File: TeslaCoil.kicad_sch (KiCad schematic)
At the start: 36 parts, among them J1 Screw_Terminal_01x03, J2 Screw_Terminal_01x02, J3 Screw_Terminal_01x02, Q1 Q_NIGBT_GCE, Q2 Q_NIGBT_GCE, U1 UCC27712D, U2 L78L15_SO8, U3 ZC323000, U4 HT7533-1-SOT89

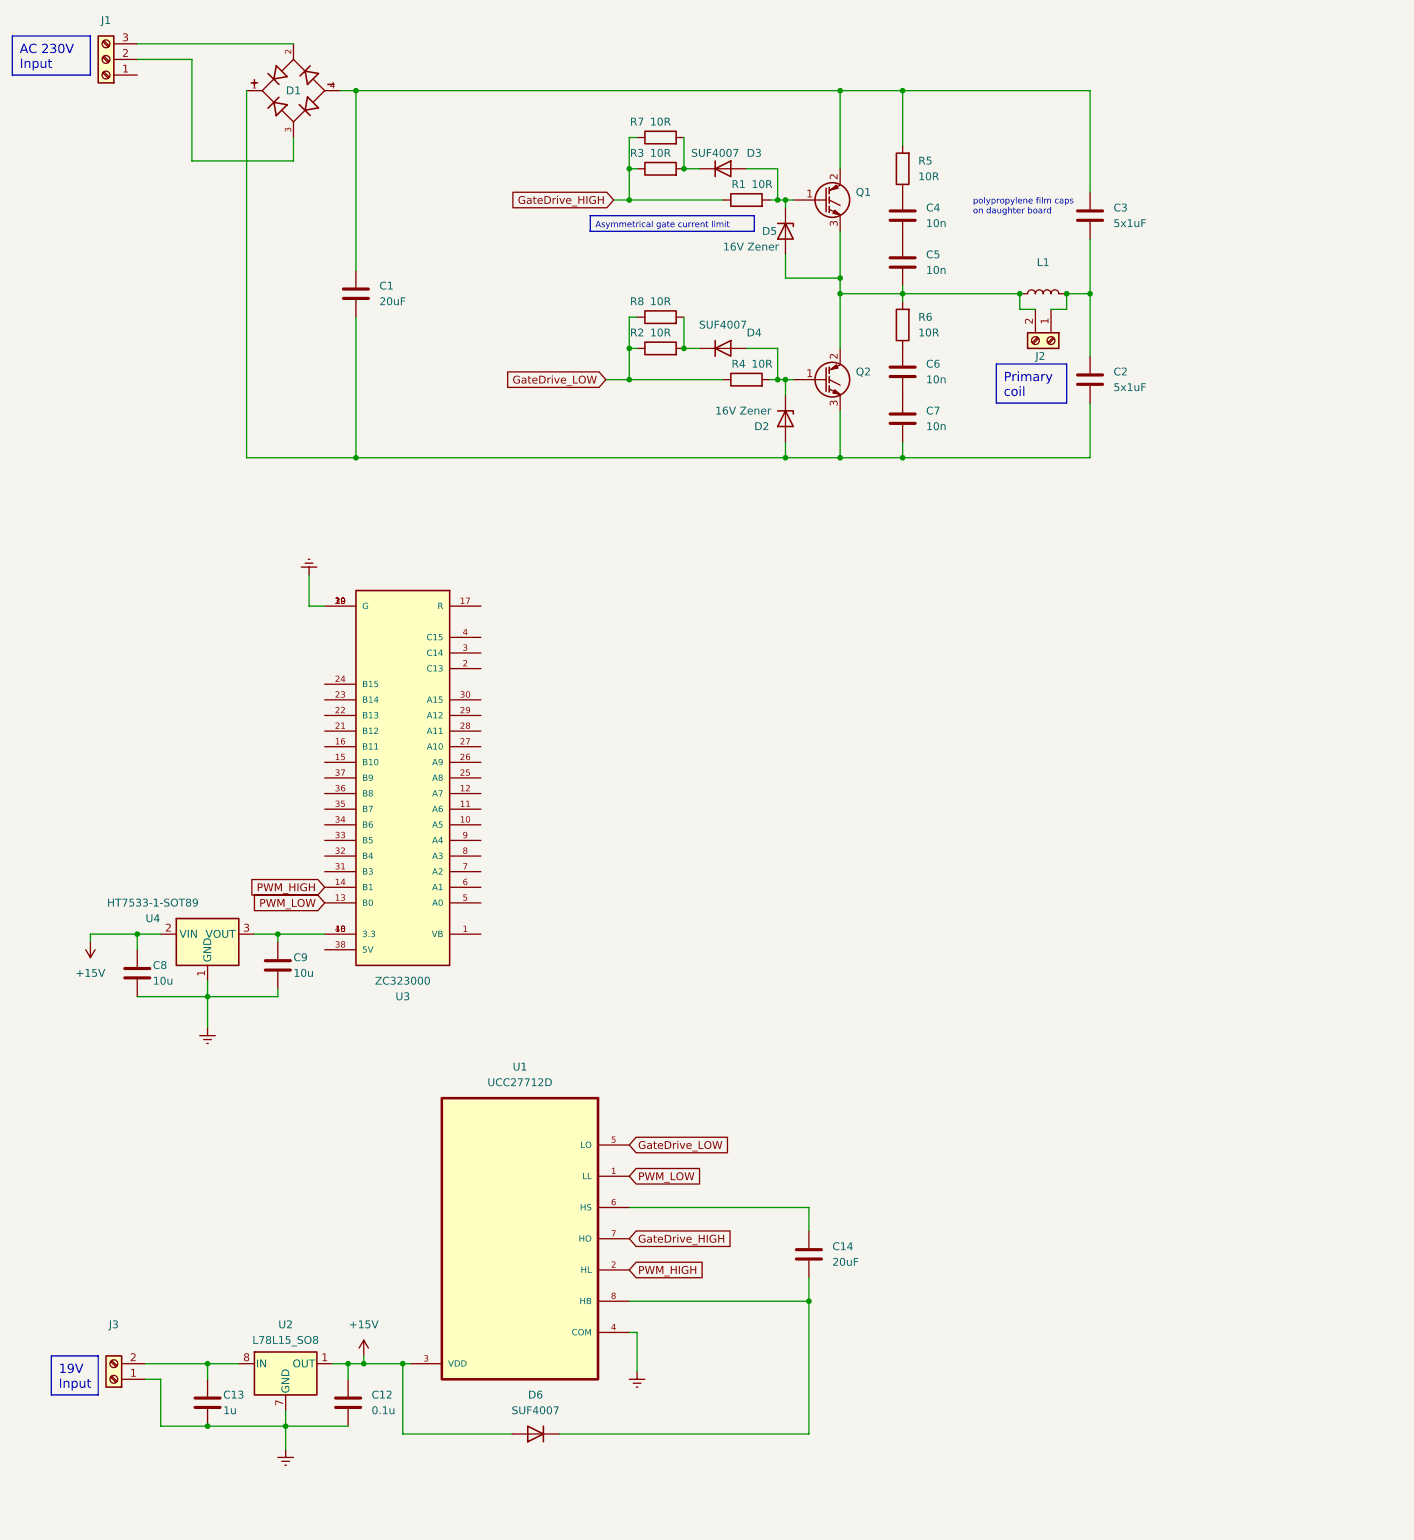
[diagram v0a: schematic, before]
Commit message: layout mockup
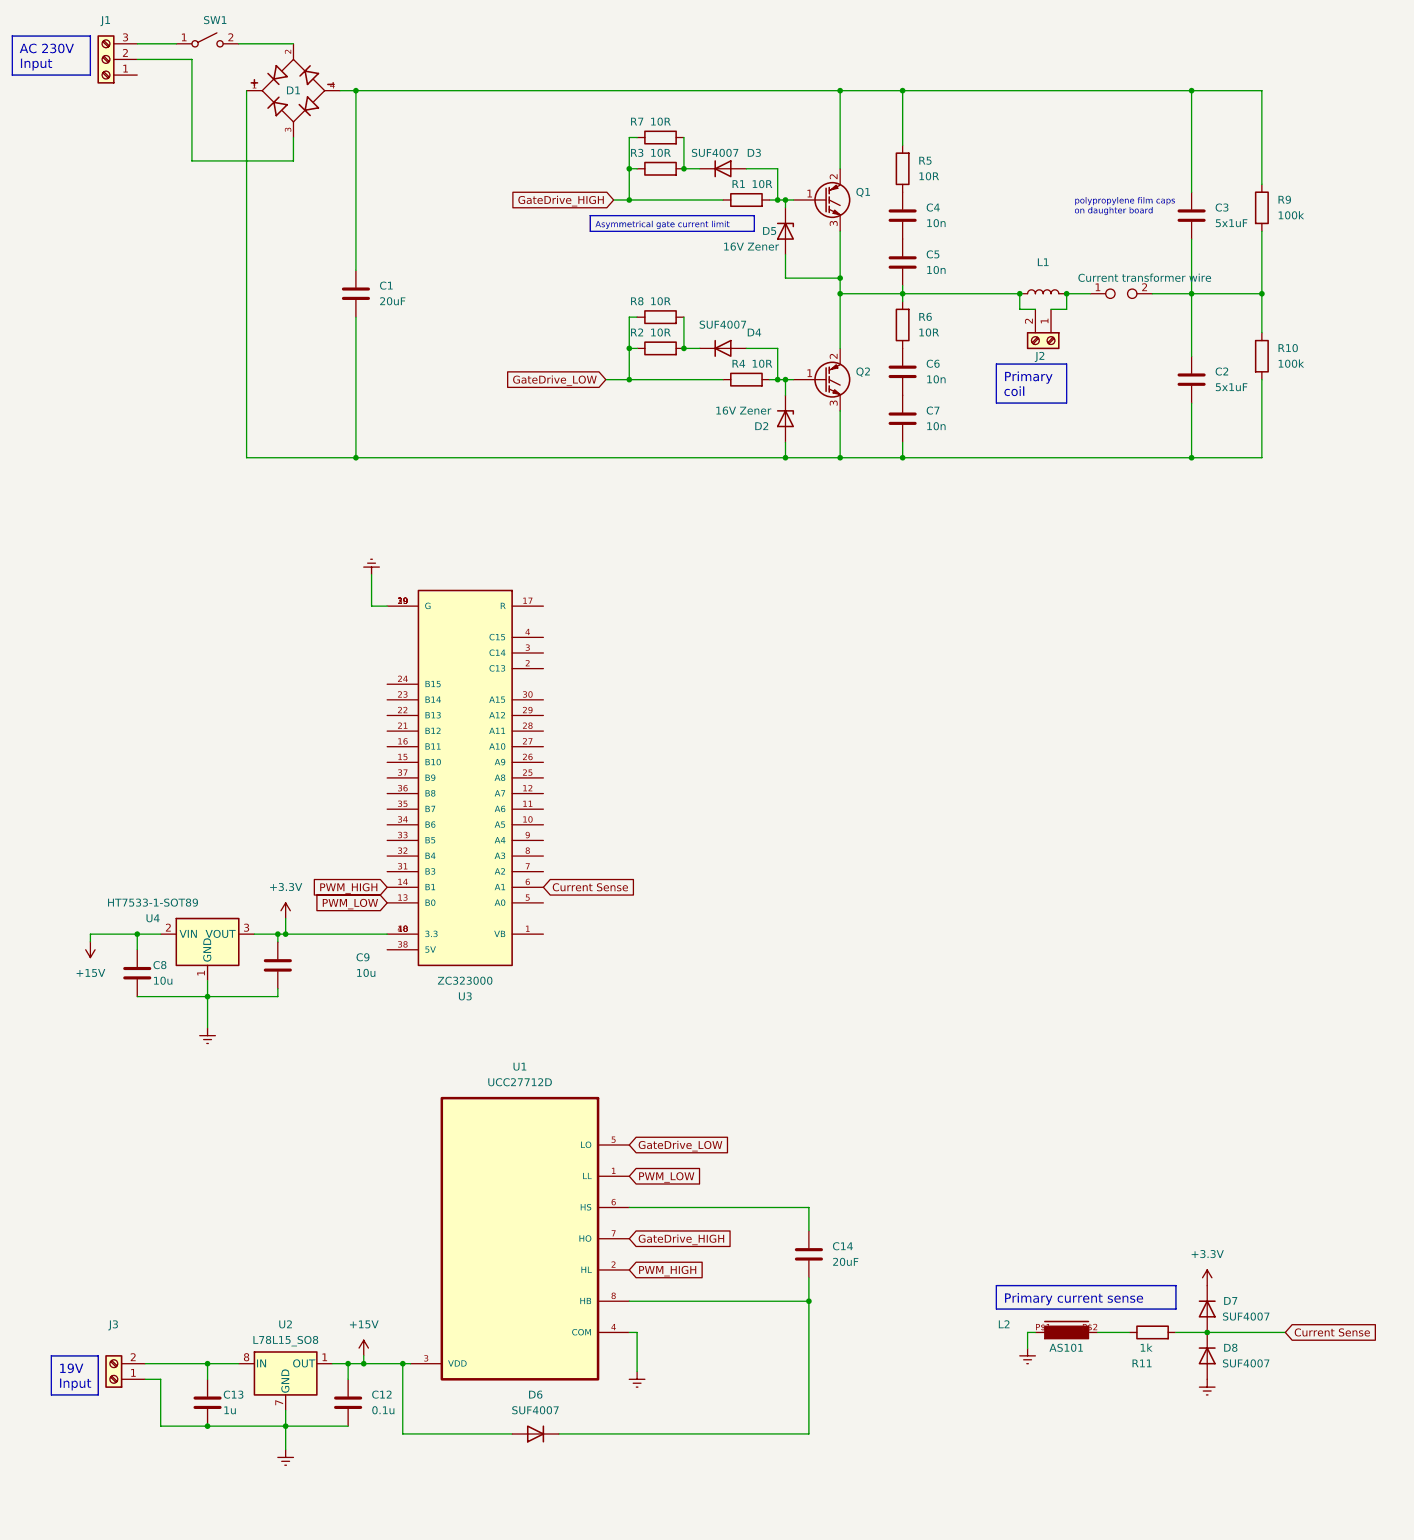
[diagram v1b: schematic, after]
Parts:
- added D7, D8: SUF4007, Diode_SMD:D_MELF_Handsoldering, symbol Diode:SM516
- added L2: AS101, Snapeda:ASM-010_ASM-010, symbol Snapeda_kicad_sym:ASM-010
- added R10, R9: 100k, Resistor_THT:R_Axial_DIN0207_L6.3mm_D2.5mm_P7.62mm_Horizontal, symbol Device:R
- added R11: 1k, Resistor_THT:R_Axial_DIN0207_L6.3mm_D2.5mm_P7.62mm_Horizontal, symbol Device:R
- added SW1: SW_SPST, symbol Switch:SW_SPST
- added TP1: Current transformer wire, TestPoint:TestPoint_Bridge_Pitch7.62mm_Drill1.3mm, symbol Connector:TestPoint_2Pole
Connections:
- net Earth: now also D8.2 (A), L2.P$1
- net at C1.2, C2.2, C7.2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: now also R10.2
- net at D1.2: now also SW1.2 (B); no longer J1.3 (Pin_3)
- net at C1.1, C3.1, D1.4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: now also R9.1
- net +3.3V: now reaches C9.1, U3.18 (3.3), U3.40 (3.3), U4.3 (VOUT)
- net +3.3V: now also D7.1 (K)
- net at J2.1 (Pin_1), L1.2: now also TP1.1; no longer C2.1, C3.2
- net Current Sense: now reaches U3.6 (A1)
- net Current Sense: now also D7.2 (A), D8.1 (K), R11.2
- new net: L2.P$2, R11.1
- new net: C2.1, C3.2, R10.1, R9.2, TP1.2
- new net: J1.3 (Pin_3), SW1.1 (A)
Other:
- moved on the sheet: C2, C3, U3

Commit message: layout 2nd rev
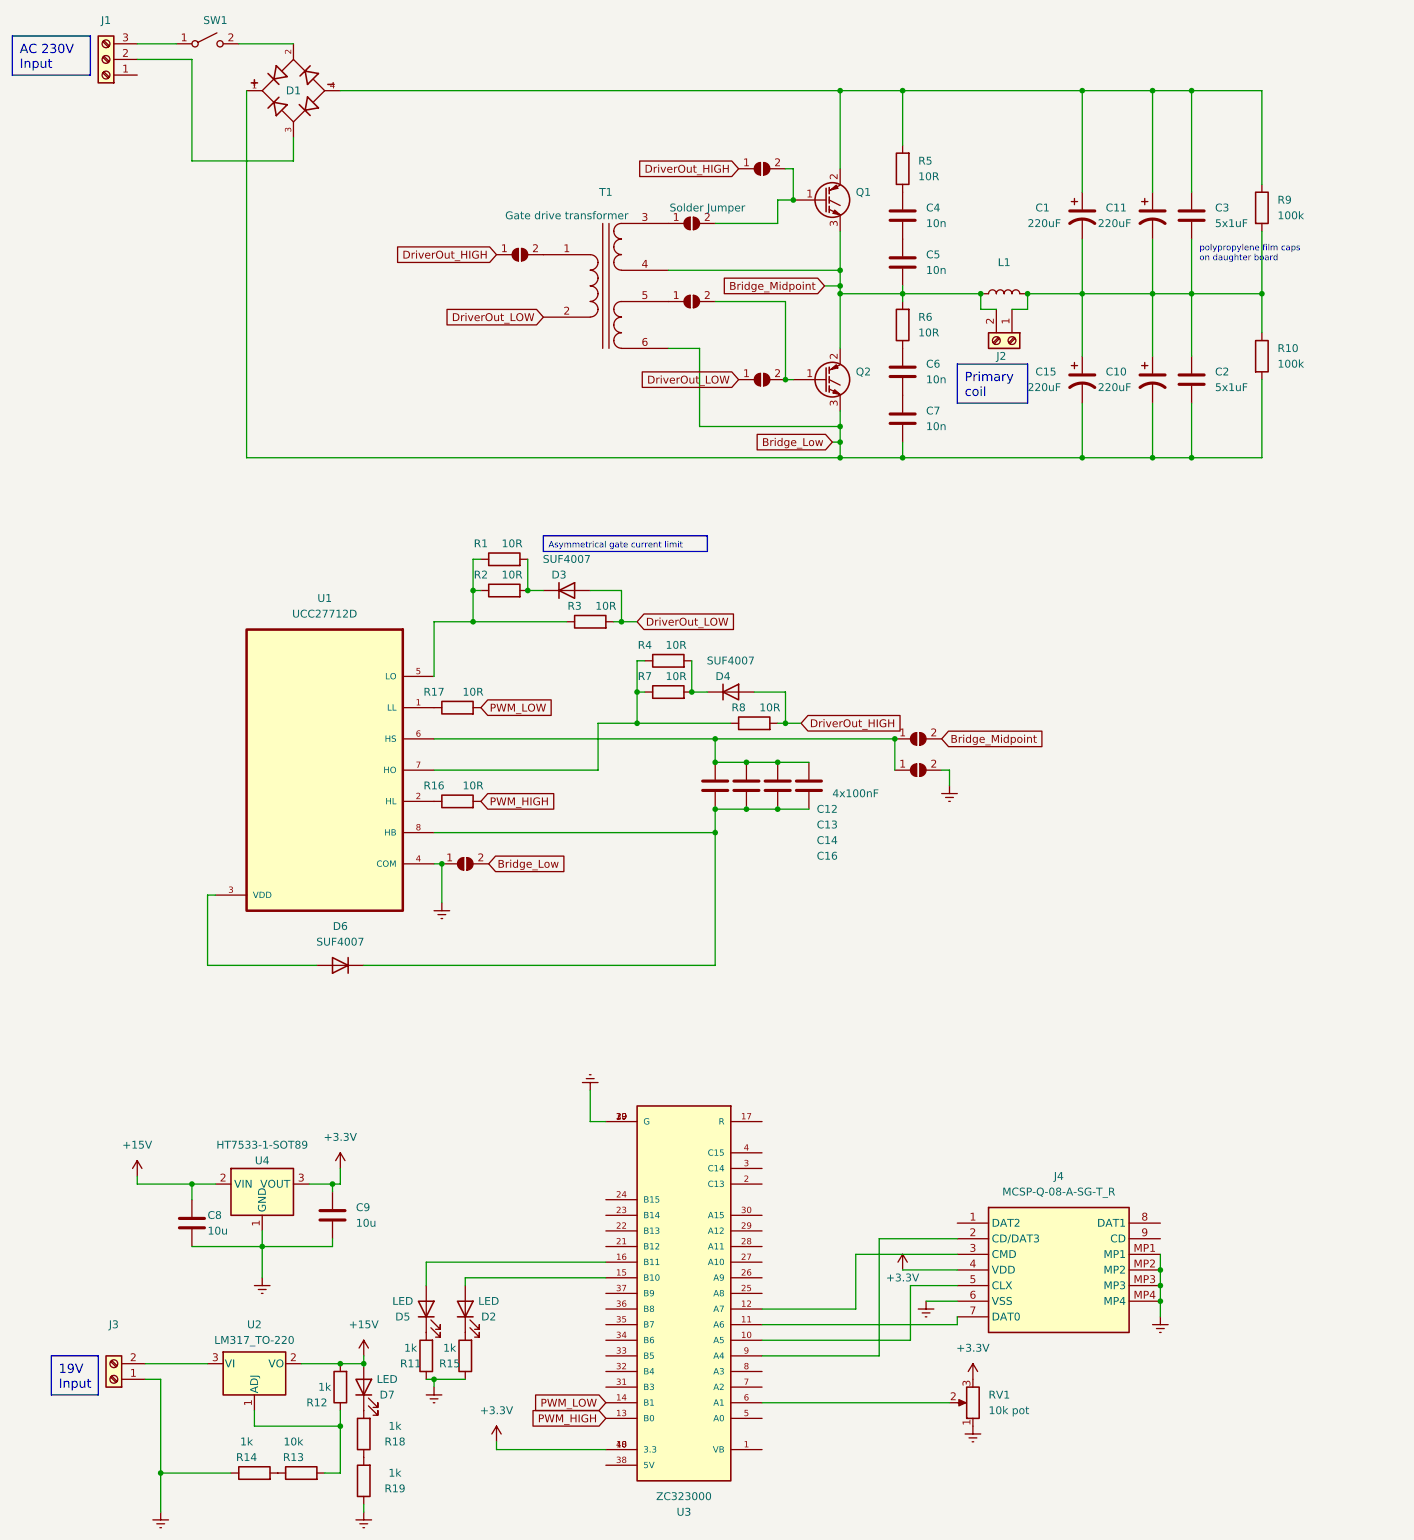
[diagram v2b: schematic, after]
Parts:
- removed C1: 20uF, Capacitor_THT:CP_Radial_D17.0mm_P7.50mm, symbol Device:C
- removed D2, D5: 16V Zener, Diode_SMD:D_0805_2012Metric, symbol Device:D_Zener
- removed D7, D8: SUF4007, Diode_SMD:D_MELF_Handsoldering, symbol Diode:SM516
- removed L2: AS101, Snapeda:ASM-010_ASM-010, symbol Snapeda_kicad_sym:ASM-010
- removed TP1: Current transformer wire, TestPoint:TestPoint_Bridge_Pitch7.62mm_Drill1.3mm, symbol Connector:TestPoint_2Pole
- removed U2: L78L15_SO8, Package_SO:SOIC-8_3.9x4.9mm_P1.27mm, symbol Regulator_Linear:L78L15_SO8
- added C1, C10, C11, C15: 220uF, Capacitor_THT:CP_Radial_D22.0mm_P10.00mm_SnapIn, symbol Device:C_Polarized_US
- added C16: 4x100nF, Capacitor_SMD:C_0603_1608Metric, symbol Device:C
- added D2, D5, D7: LED, LED_SMD:LED_0805_2012Metric, symbol Device:LED
- added J4: MCSP-Q-08-A-SG-T_R, Samacsys:MCSPQ08ASGTR, symbol Samacsys_kicad_sym:MCSP-Q-08-A-SG-T_R
- added JP1, JP2, JP3, JP4, JP5, JP6, JP7, JP8: Solder Jumper, Jumper:SolderJumper-2_P1.3mm_Open_TrianglePad1.0x1.5mm, symbol Jumper:SolderJumper_2_Open
- added R12, R14, R15, R18, R19: 1k, Resistor_SMD:R_0603_1608Metric_Pad0.98x0.95mm_HandSolder, symbol Device:R
- added R13: 10k, Resistor_SMD:R_0603_1608Metric_Pad0.98x0.95mm_HandSolder, symbol Device:R
- added R16, R17: 10R, Resistor_SMD:R_0603_1608Metric_Pad0.98x0.95mm_HandSolder, symbol Device:R
- added RV1: 10k pot, Snapeda:potentiometer, symbol Device:R_Potentiometer
- added T1: Gate drive transformer, Transformer_THT:Transformer_Toroid_Tapped_Horizontal_D10.5mm_Amidon-T37, symbol Device:Transformer_1P_2S
- added U2: LM317_TO-220, Package_TO_SOT_THT:TO-220-3_Vertical, symbol Regulator_Linear:LM317_TO-220
- C12: value 0.1u -> 100nF; footprint Capacitor_SMD:C_0805_2012Metric_Pad1.18x1.45mm_HandSolder -> Capacitor_SMD:C_0603_1608Metric
- C13: value 1u -> 100nF; footprint Capacitor_SMD:C_0805_2012Metric_Pad1.18x1.45mm_HandSolder -> Capacitor_SMD:C_0603_1608Metric
- C14: value 20uF -> 100nF; footprint Capacitor_SMD:C_0805_2012Metric_Pad1.18x1.45mm_HandSolder -> Capacitor_SMD:C_0603_1608Metric
- R11: footprint Resistor_THT:R_Axial_DIN0207_L6.3mm_D2.5mm_P7.62mm_Horizontal -> Resistor_SMD:R_0603_1608Metric_Pad0.98x0.95mm_HandSolder
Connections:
- net +15V: now also D7.2 (A), R12.2, U2.2 (VO); no longer C12.1, D6.2 (A), U1.3 (VDD)
- net +3.3V: now also J4.4 (VDD), RV1.3
- net Earth: now also R11.1, J4.6 (VSS), J4.MP1, J4.MP2, J4.MP3, J4.MP4, JP7.2 (B), JP8.1 (A), R14.1, R15.1, R19.1, RV1.1; no longer C12.2, C13.2
- net PWM_HIGH: now also U3.13 (B0), R16.2; no longer U1.2 (HL), U3.14 (B1)
- net PWM_LOW: now also U3.14 (B1), R17.2; no longer U1.1 (LL), U3.13 (B0)
- net at J3.2 (Pin_2): now also U2.3 (VI); no longer C13.1
- net Bridge_Low: now reaches C2.2, C7.2, D1.1, Q2.3 (E), R10.2
- net Bridge_Low: now also C10.2, C15.2, JP8.2 (B), T1.6 (SD)
- net at C3.1, D1.4, Q1.2 (C)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: now also C1.1, C11.1
- net Bridge_Midpoint: now reaches C5.2, J2.2 (Pin_2), L1.1, Q1.3 (E), Q2.2 (C), R6.2
- net Bridge_Midpoint: now also JP6.2 (B), T1.4 (SB)
- net at C14.2, D6.1 (K), U1.8 (HB): now also C12.2, C13.2, C16.2
- net at C14.1, U1.6 (HS): now also C12.1, C13.1, C16.1, JP6.1 (A), JP7.1 (A)
- net at J2.1 (Pin_1), L1.2: now also C2.1, C3.2, R10.1, R9.2, C1.2, C10.1, C11.2, C15.1
- net at U3.10 (A5): now also J4.5 (CLX)
- net at U3.11 (A6): now also J4.7 (DAT0)
- net at U3.12 (A7): now also J4.3 (CMD)
- net at U3.15 (B10): now also D2.2 (A)
- net at U3.16 (B11): now also D5.2 (A)
- net at U3.9 (A4): now also J4.2 (CD/DAT3)
- net Current Sense: no longer names the net of U3.6 (A1)
- net Current Sense: now also RV1.2; no longer R11.2
- net GateDrive_HIGH: no longer names the net of R7.1, U1.7 (HO)
- net GateDrive_HIGH: now also R4.1, R8.1; no longer R1.1, R3.1
- net GateDrive_LOW: no longer names the net of R2.1, U1.5 (LO)
- net GateDrive_LOW: now also R1.1, R3.1; no longer R4.1, R8.1
- new net: R13.1, R14.2
- new net: R12.1, R13.2, U2.1 (ADJ)
- new net: R18.1, R19.2
- new net: D7.1 (K), R18.2
- new net: D3.1 (K), R1.2, R2.2
- new net: R17.1, U1.1 (LL)
- new net: JP1.1 (A), T1.3 (SA)
- new net: JP1.2 (B), JP5.2 (B), Q1.1 (G)
- new net: JP2.2 (B), JP4.2 (B), Q2.1 (G)
- new net: D2.1 (K), R15.2
- new net: D6.2 (A), U1.3 (VDD)
- new net: R16.1, U1.2 (HL)
- new net: JP3.2 (B), T1.1 (AA)
- new net: JP2.1 (A), T1.5 (SC)
- new net: D5.1 (K), R11.2
- new net: D4.1 (K), R4.2, R7.2
- new net DriverOut_HIGH: D4.2 (A), JP3.1 (A), JP5.1 (A), R8.2
- new net DriverOut_LOW: D3.2 (A), JP4.1 (A), R3.2, T1.2 (AB)
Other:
- moved on the sheet: C14, C8, C9, D6, J2, L1, U1, U3, U4
